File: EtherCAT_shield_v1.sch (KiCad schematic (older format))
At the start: 20 parts, among them J1 RJ45-PULSETRANS, J2 RJ45-PULSETRANS, P1 CONN_02X10, P2 CONN_02X19, P3 CONN_02X19, U1 LAN9252

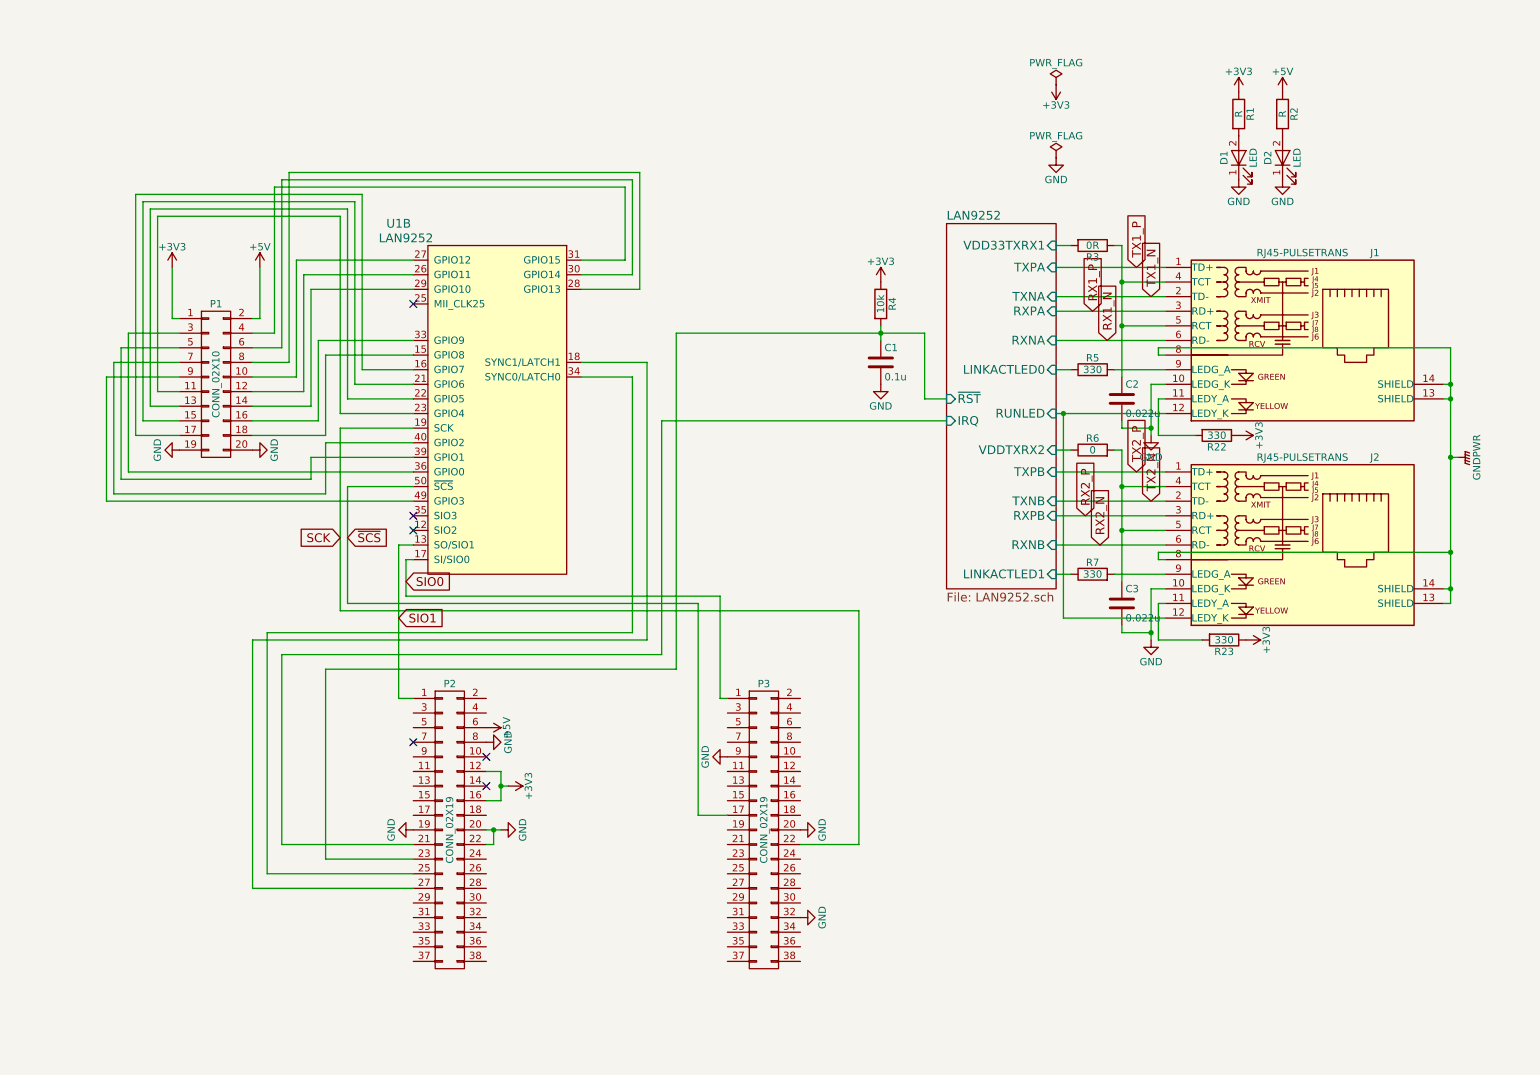
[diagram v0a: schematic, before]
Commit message: GPIOのLED並べた 実質完成
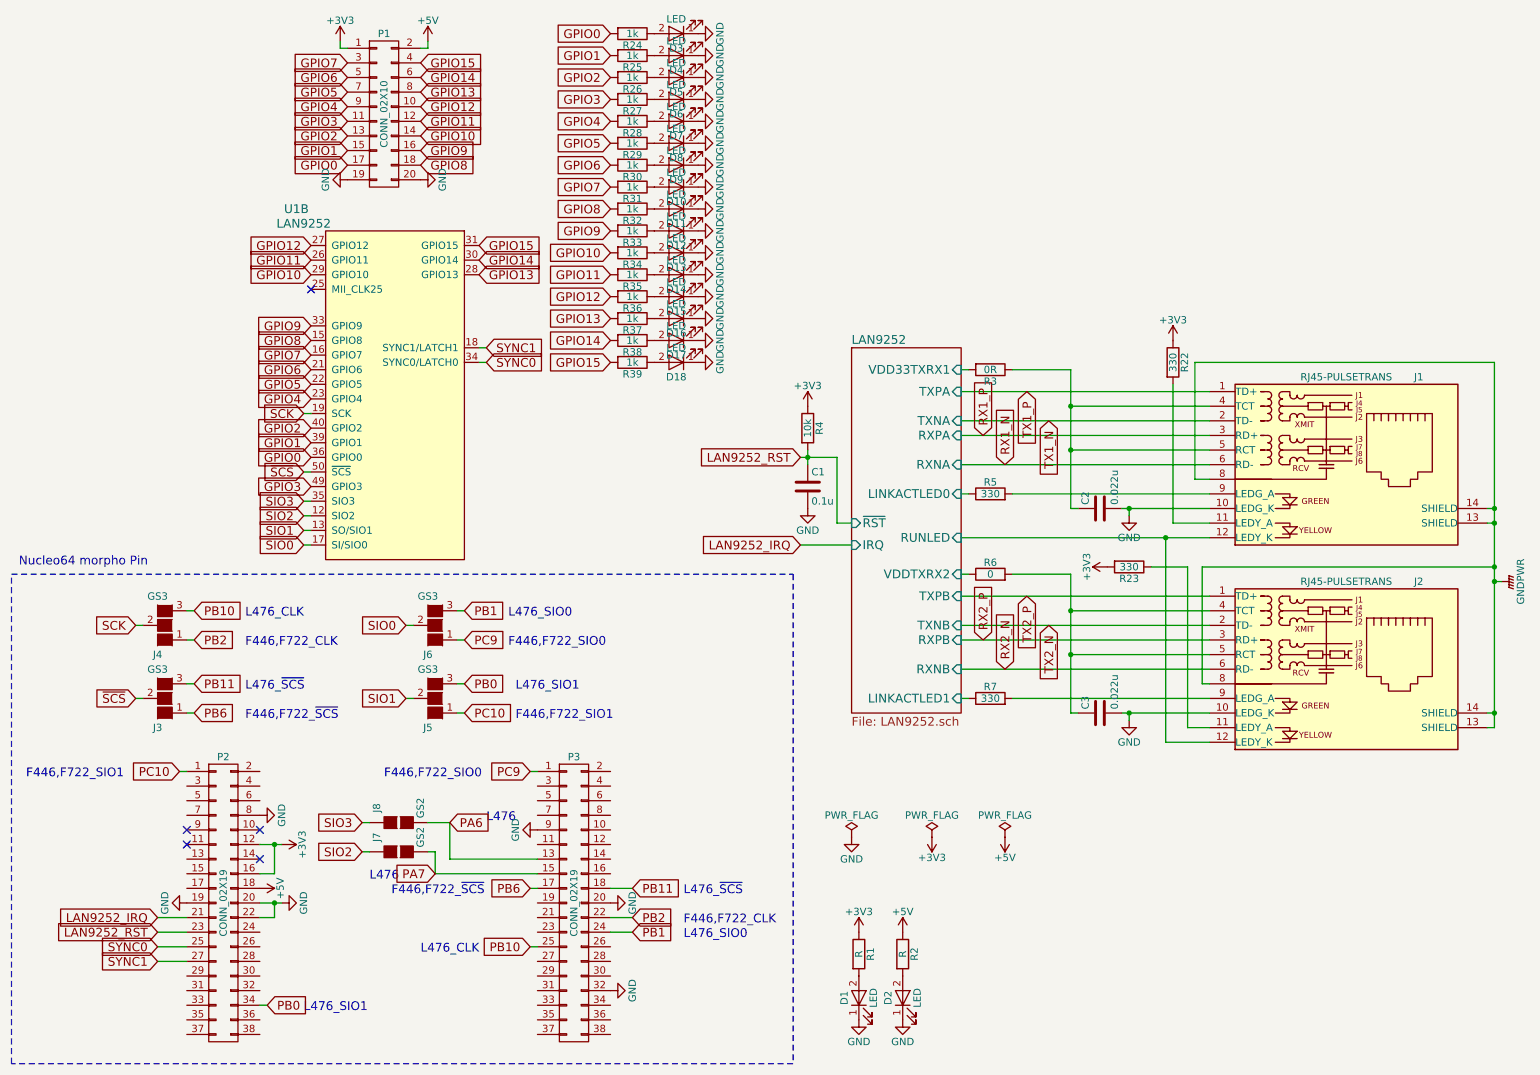
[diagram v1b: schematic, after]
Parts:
- added D10, D11, D12, D13, D14, D15, D16, D17, D18, D3, D4, D5, D6, D7, D8, D9: LED, LEDs:LED_0603, symbol LED
- added J3, J4, J5, J6: GS3, Connect:GS3, symbol GS3
- added J7, J8: GS2, Connect:GS2, symbol GS2
- added R24, R25, R26, R27, R28, R29, R30, R31, R32, R33, R34, R35, R36, R37, R38, R39: 1k, Resistors_SMD:R_0603, symbol R
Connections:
- net +3V3: now also R23.2; no longer R23.1
- net +5V: now also P2.18 (P18); no longer P2.6 (P6)
- net GND: now also D10.1 (K), D11.1 (K), D12.1 (K), D13.1 (K), D14.1 (K), D15.1 (K), D16.1 (K), D17.1 (K), D18.1 (K), D3.1 (K), D4.1 (K), D5.1 (K), D6.1 (K), D7.1 (K), D8.1 (K), D9.1 (K)
- net SCK: now also J4.2 (G2); no longer P3.22 (P22)
- net SIO0: now also J6.2 (G2); no longer P3.1 (P1)
- net SIO1: now also J5.2 (G2); no longer P2.1 (P1)
- net ~SCS: now also J3.2 (G2); no longer P3.17 (P17)
- net at J2.11 (LEDY_A): now also R23.1; no longer R23.2
- net SIO2: now reaches U1.12 (SIO2)
- net SIO2: now also J7.1 (G1)
- net GPIO8: now reaches P1.18 (P18), U1.15 (GPIO8)
- net GPIO8: now also R32.2
- net GPIO0: now reaches P1.17 (P17)
- net GPIO0: now also U1.36 (GPIO0), R24.2; no longer U1.16 (GPIO7)
- net SYNC1: now reaches P2.27 (P27), U1.18 (SYNC1/LATCH1)
- net GPIO1: now reaches P1.15 (P15)
- net GPIO1: now also U1.39 (GPIO1), R25.2; no longer U1.21 (GPIO6)
- net GPIO2: now reaches P1.13 (P13)
- net GPIO2: now also U1.40 (GPIO2), R26.2; no longer U1.22 (GPIO5)
- net GPIO3: now reaches P1.11 (P11)
- net GPIO3: now also U1.49 (GPIO3), R27.2; no longer U1.23 (GPIO4)
- net GPIO11: now reaches P1.12 (P12), U1.26 (GPIO11)
- net GPIO11: now also R35.2
- net GPIO12: now reaches P1.10 (P10), U1.27 (GPIO12)
- net GPIO12: now also R36.2
- net GPIO13: now reaches P1.8 (P8), U1.28 (GPIO13)
- net GPIO13: now also R37.2
- net GPIO10: now reaches P1.14 (P14), U1.29 (GPIO10)
- net GPIO10: now also R34.2
- net GPIO14: now reaches P1.6 (P6), U1.30 (GPIO14)
- net GPIO14: now also R38.2
- net GPIO15: now reaches P1.4 (P4), U1.31 (GPIO15)
- net GPIO15: now also R39.2
- net GPIO9: now reaches P1.16 (P16), U1.33 (GPIO9)
- net GPIO9: now also R33.2
- net SYNC0: now reaches P2.25 (P25), U1.34 (SYNC0/LATCH0)
- net SIO3: now reaches U1.35 (SIO3)
- net SIO3: now also J8.1 (G1)
- net GPIO7: now reaches P1.3 (P3)
- net GPIO7: now also U1.16 (GPIO7), R31.2; no longer U1.36 (GPIO0)
- net GPIO6: now reaches P1.5 (P5)
- net GPIO6: now also U1.21 (GPIO6), R30.2; no longer U1.39 (GPIO1)
- net GPIO5: now reaches P1.7 (P7)
- net GPIO5: now also U1.22 (GPIO5), R29.2; no longer U1.40 (GPIO2)
- net GPIO4: now reaches P1.9 (P9)
- net GPIO4: now also U1.23 (GPIO4), R28.2; no longer U1.49 (GPIO3)
- net PB0: now reaches P2.34 (P34)
- net PB0: now also J5.3 (G3)
- net PA6: now reaches P3.13 (P13)
- net PA6: now also J8.2 (G2)
- net PA7: now reaches P3.15 (P15)
- net PA7: now also J7.2 (G2)
- net PB11: now reaches P3.18 (P18)
- net PB11: now also J3.3 (G3)
- net PB1: now reaches P3.24 (P24)
- net PB1: now also J6.3 (G3)
- net PB10: now reaches P3.25 (P25)
- net PB10: now also J4.3 (G3)
- net LAN9252/IRQ renamed LAN9252_IRQ
- net LAN9252/~RST renamed LAN9252_RST
- new net: D3.2 (A), R24.1
- new net: D4.2 (A), R25.1
- new net: D5.2 (A), R26.1
- new net: D6.2 (A), R27.1
- new net: D7.2 (A), R28.1
- new net: D8.2 (A), R29.1
- new net: D9.2 (A), R30.1
- new net: D10.2 (A), R31.1
- new net: D11.2 (A), R32.1
- new net: D12.2 (A), R33.1
- new net: D13.2 (A), R34.1
- new net: D14.2 (A), R35.1
- new net: D15.2 (A), R36.1
- new net: D16.2 (A), R37.1
- new net: D17.2 (A), R38.1
- new net: D18.2 (A), R39.1
- new net PB2: J4.1 (G1), P3.22 (P22)
- new net PB6: J3.1 (G1), P3.17 (P17)
- new net PC10: J5.1 (G1), P2.1 (P1)
- new net PC9: J6.1 (G1), P3.1 (P1)
- no-connect marks 6 -> 5
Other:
- note added: "F446,F722_CLK"
- note added: "F446,F722_SIO0"
- note added: "F446,F722_SIO1"
- note added: "F446,F722_~SCS"
- note added: "L476"
- note added: "L476_CLK"
- note added: "L476_SIO0"
- note added: "L476_SIO1"
- note added: "L476_~SCS"
- note added: "Nucleo64 morpho Pin"
- moved on the sheet: C1, C2, C3, D1, D2, J1, J2, P1, P2, P3, R1, R2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
